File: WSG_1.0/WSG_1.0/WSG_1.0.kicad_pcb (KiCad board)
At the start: 4 copper layers, 68.8 x 27.7 mm, 123 parts, among them J1 Conn_01x10, J2 USB_C_Receptacle_USB2.0_16P, J4 Conn_01x02, SW3 SW_Push, SW4 SW_Push, U1 ADS131A04IPBSR, U10 TPS22916CYFPR, U11 W25N04KVZEIR, U12 USBLC6-2SC6, U14 TPD4E1U06DBVR, U15 ESP32-S3-MINI-1U-N8, U2 DAC60501ZDGSR, U3 INA827AIDGKR, U4 INA827AIDGKR, U5 INA827AIDGKR, U6 TMP235A2DBZR, U7 BQ25180YBGR, U8 TPS63802DLAR, U9 TPS7A2025PDBVR, Y1 SiT8008AI-12-33S-16.384000

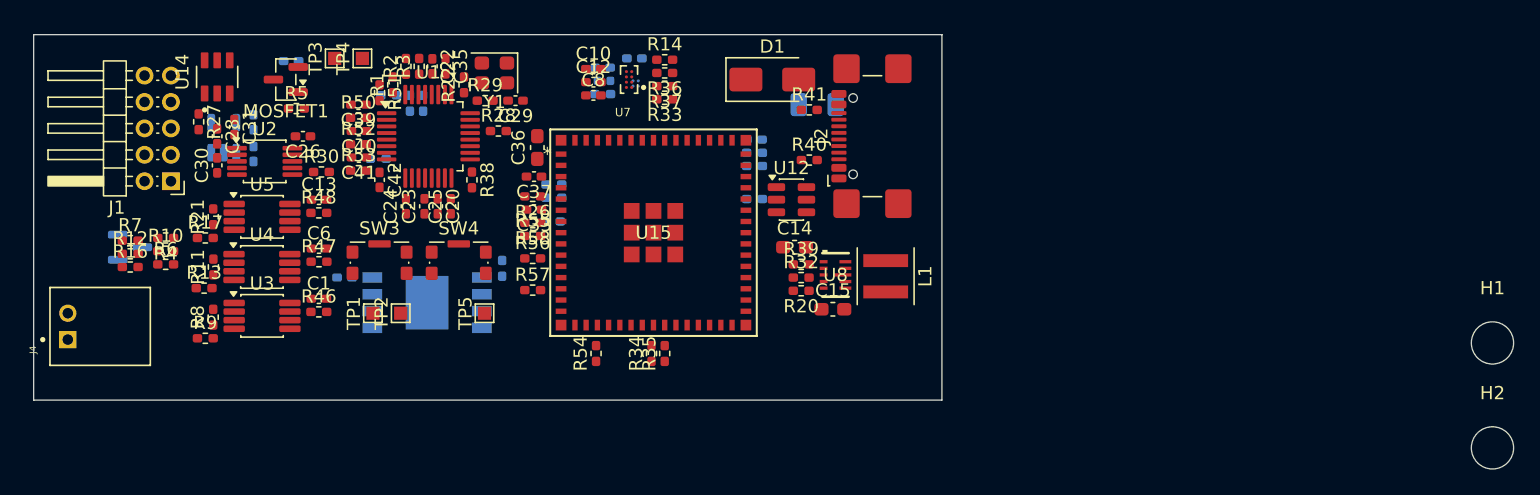
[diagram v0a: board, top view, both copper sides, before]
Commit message: ~1/2 done with routing, neeed to undo some
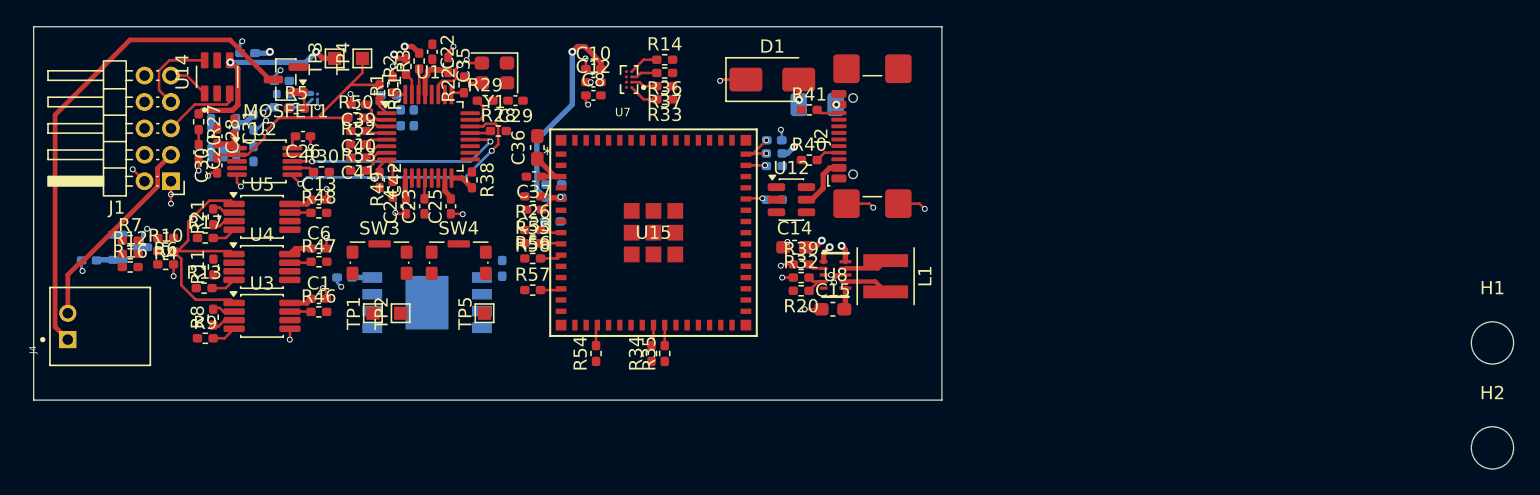
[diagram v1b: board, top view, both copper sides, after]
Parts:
- R49: moved to F.Cu
- moved C2 29.3 mm to (102.5, 62.8)
- moved C34 24.3 mm to (105.1, 64.9)
- moved R24 24.3 mm to (105.1, 66.9)
- moved U10 24.3 mm to (107.6, 66.1)
- moved FB1 24.3 mm to (105.2, 65.9)
- moved C21 21.5 mm to (90.5, 78.5)
- moved C20 18.6 mm to (98.8, 70.3)
- moved R49 2.55 mm to (113.5, 73.1), turned to 90 degrees
- moved C38 1.50 mm to (142.4, 69.4)
- moved R43 1.50 mm to (142.4, 73.9)
- moved R45 1.50 mm to (142.4, 70.4)
- moved R44 1.50 mm to (142.4, 71.3)
- moved R15 1.31 mm to (115.1, 67.7)
- moved R18 1.31 mm to (114.1, 67.7)
- moved C22 1.10 mm to (116.5, 62.7)
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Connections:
- C20 pad 1: REFEXT_F -> Net-(C20-Pad1)
- R27 pad 2: REFEXT_F -> Net-(C20-Pad1)
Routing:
- net GND: track 0.00 -> 42.1 mm, vias 0 -> 40
- net BATT_P: track 0.00 -> 37.6 mm
- net VREF_1V65: track 0.00 -> 22.8 mm, vias 0 -> 1
- net 3V3A: track 0.00 -> 21.7 mm, vias 0 -> 3
- net ADC_SCLK: track 0.00 -> 20.8 mm, vias 0 -> 2
- net BREF_F: track 0.00 -> 19.2 mm
- net ADC_MOSI: track 0.00 -> 17.2 mm, vias 0 -> 2
- net EXC_2V5: track 0.00 -> 17.0 mm, vias 0 -> 2
- net VBAT: track 0.00 -> 15.8 mm, vias 0 -> 1
- net BATT_N: track 0.00 -> 15.3 mm
- net 3V3: track 0.00 -> 8.11 mm, vias 0 -> 1
- net SIG1: track 0.00 -> 6.53 mm
- net SIG2: track 0.00 -> 5.90 mm
- net VBUS: track 0.00 -> 4.31 mm, vias 0 -> 1
- net SYS: track 0.00 -> 4.02 mm, vias 0 -> 3
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- added copper zone on In2.Cu, net 3V3
- added copper zone on In2.Cu, net 3V3A
- added copper zone on In2.Cu, net SYS
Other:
- board size 68.8 x 27.7 mm -> 68.8 x 28.3 mm
